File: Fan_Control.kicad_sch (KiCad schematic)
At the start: 34 parts, among them IC1 ADT7470ARQZ-REEL7, J1 Conn_01x04, Q3 BUK9M23-80E, Q4 BUK9M23-80E, Q5 BUK9M23-80E, Q6 BUK9M23-80E

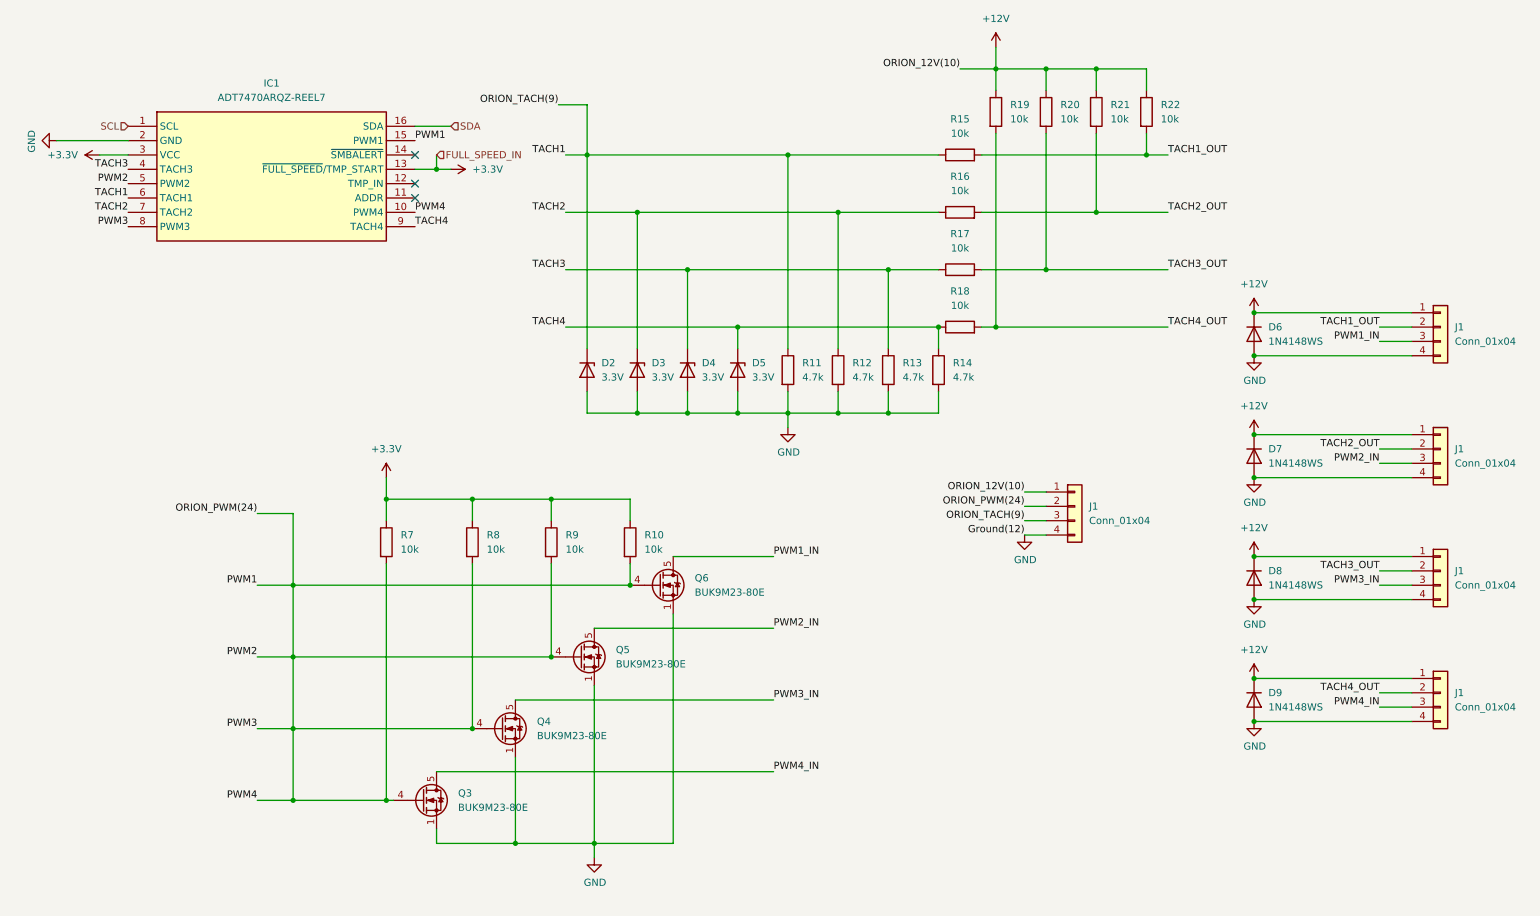
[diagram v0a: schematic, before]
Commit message: Fans-Orion Pwms isolated
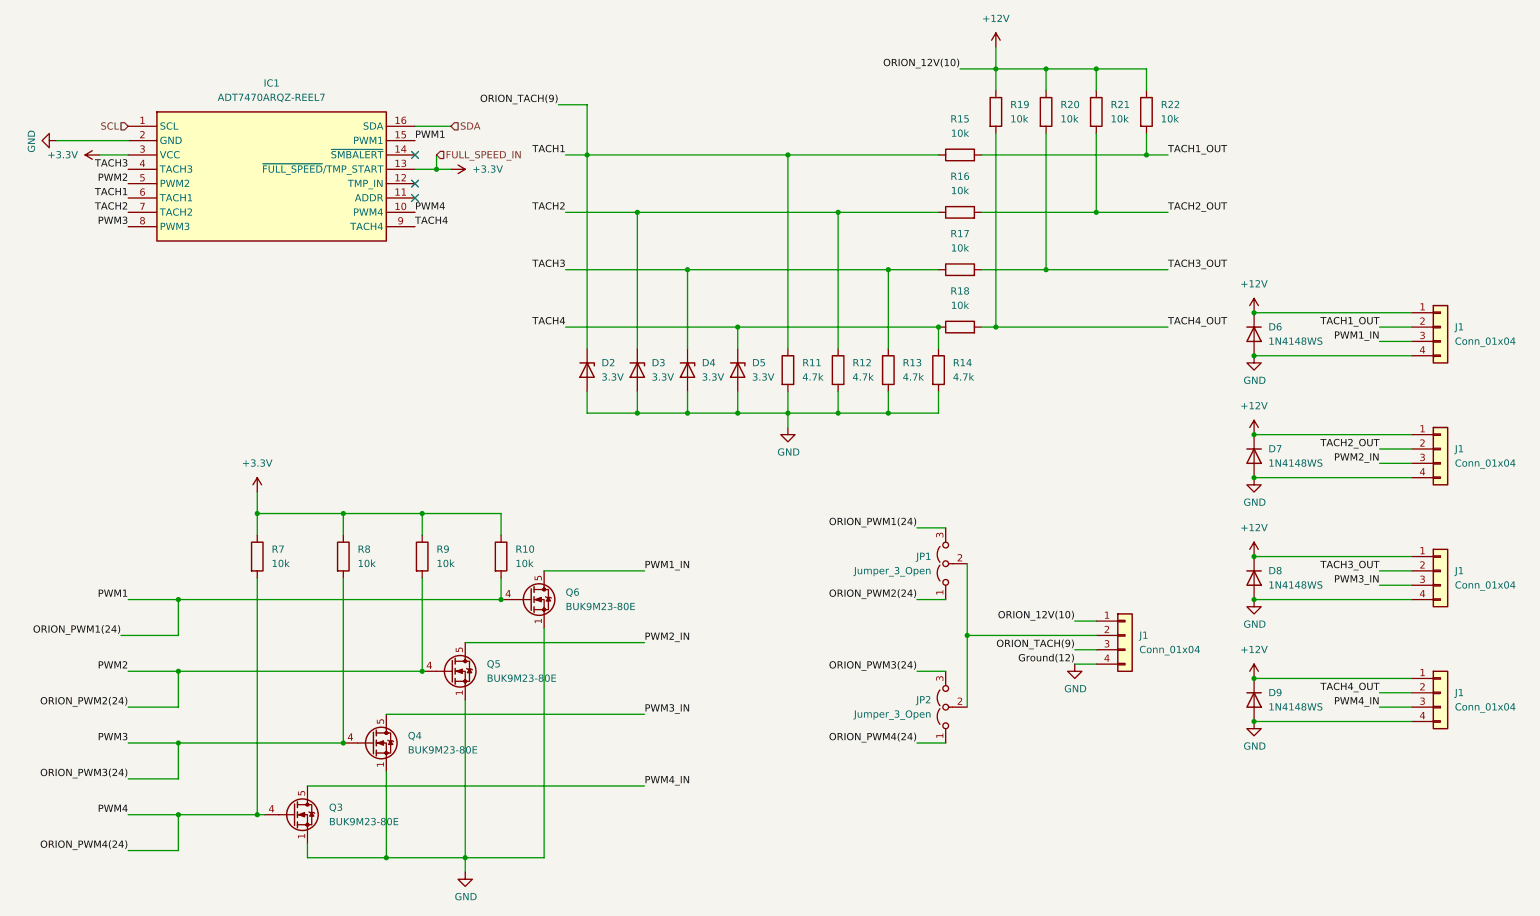
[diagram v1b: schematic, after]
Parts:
- added JP1, JP2: Jumper_3_Open, symbol Jumper:Jumper_3_Open
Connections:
- removed net ORION_PWM(24): IC1.10 (PWM4), IC1.15 (PWM1), IC1.5 (PWM2), IC1.8 (PWM3), J1.2 (Pin_2), Q3.4 (G), Q4.4 (G), Q5.4 (G), Q6.4 (G), R10.2, R7.2, R8.2, R9.2
- new net: J1.2 (Pin_2), JP1.2 (C), JP2.2 (C)
- new net ORION_PWM1(24): IC1.15 (PWM1), JP1.3 (B), Q6.4 (G), R10.2
- new net ORION_PWM2(24): IC1.5 (PWM2), JP1.1 (A), Q5.4 (G), R9.2
- new net ORION_PWM3(24): IC1.8 (PWM3), JP2.3 (B), Q4.4 (G), R8.2
- new net ORION_PWM4(24): IC1.10 (PWM4), JP2.1 (A), Q3.4 (G), R7.2
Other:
- moved on the sheet: J1, Q3, Q4, Q5, Q6, R10, R7, R8, R9
